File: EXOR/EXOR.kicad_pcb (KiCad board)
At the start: 2 copper layers, 10 parts

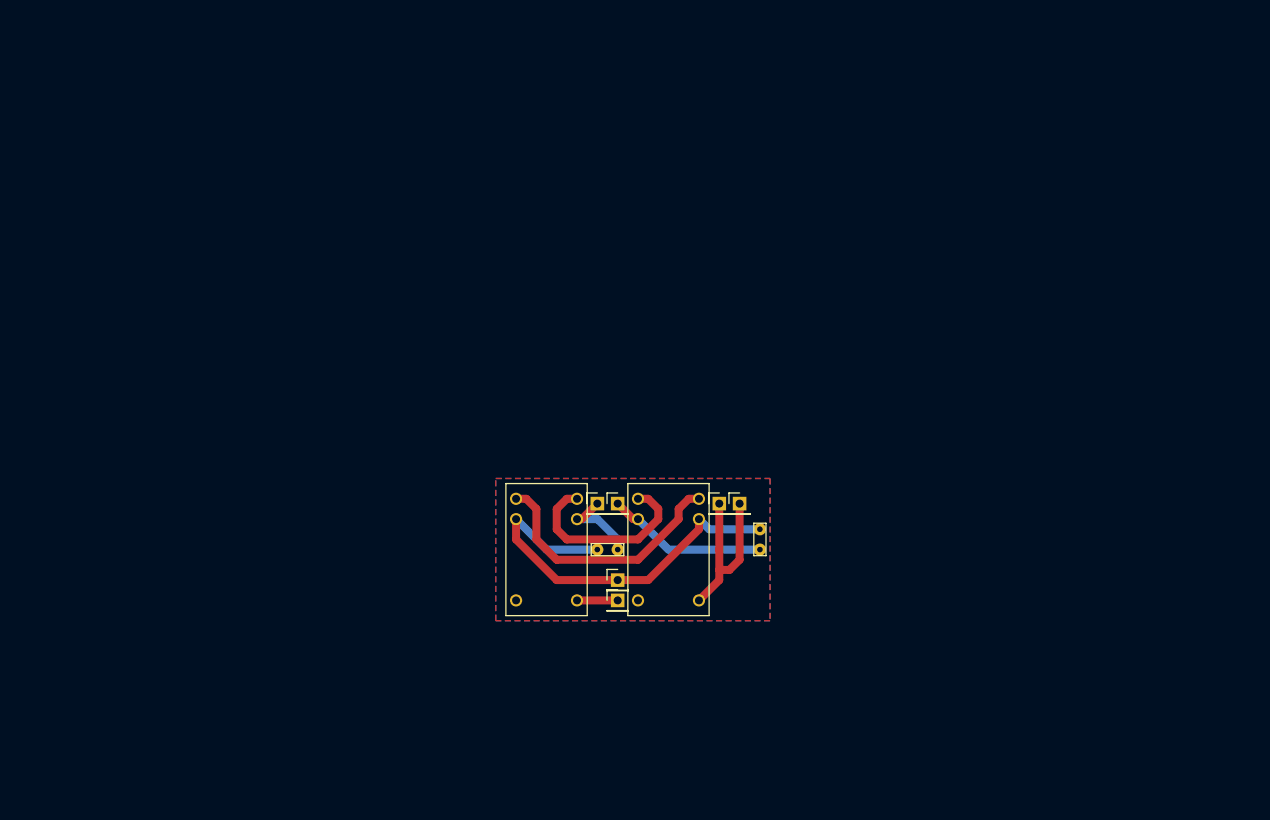
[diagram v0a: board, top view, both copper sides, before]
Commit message: Add files via upload
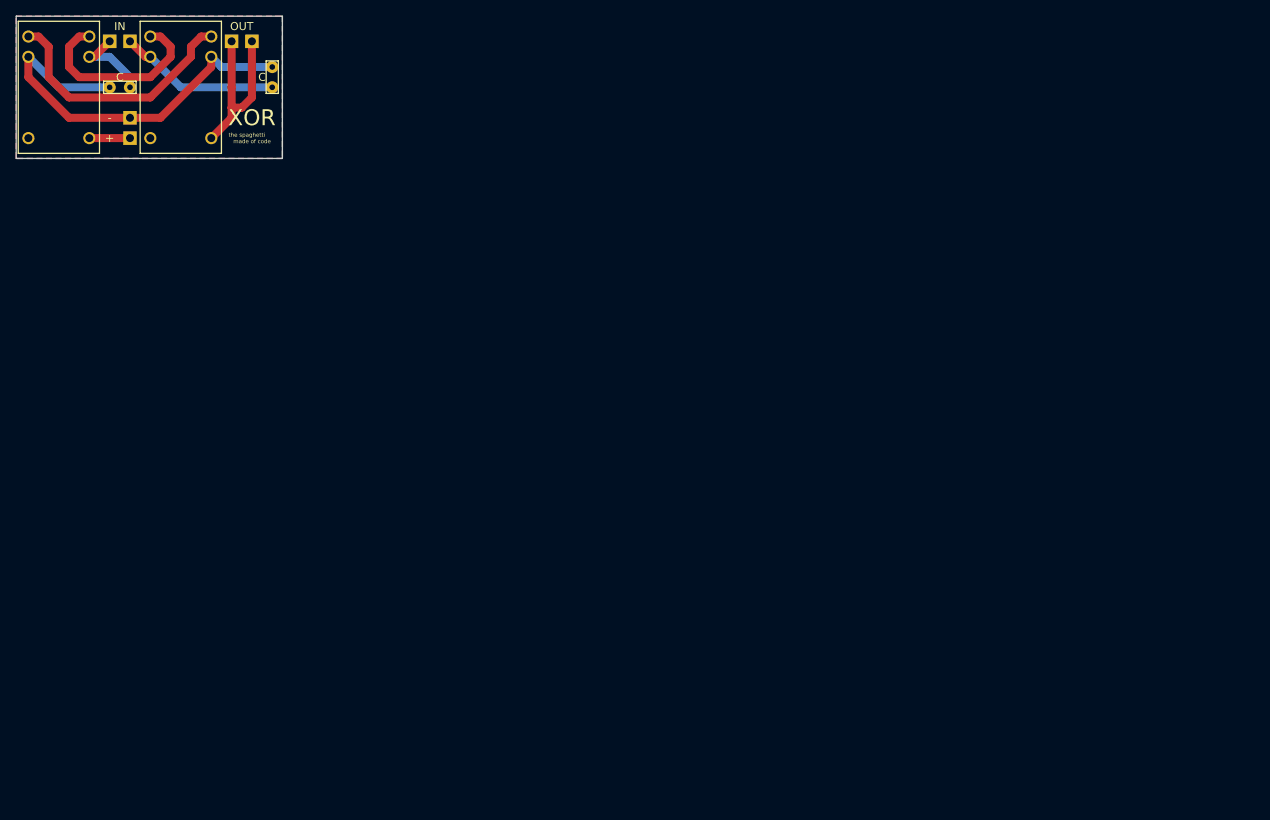
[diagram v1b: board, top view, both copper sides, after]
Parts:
- REF** (x6): moved to B.Cu
- moved REF** 84.0 mm to (45.7, 22.2)
- moved REF** 84.0 mm to (27.9, 26.0)
- moved REF** 84.0 mm to (27.9, 28.6)
- moved REF** 84.0 mm to (27.9, 16.5)
- moved REF** 84.0 mm to (20.3, 21.0)
- moved REF** 84.0 mm to (25.4, 22.2)
- moved REF** 84.0 mm to (43.2, 16.5)
- moved REF** 84.0 mm to (25.4, 16.5)
- moved REF** 84.0 mm to (40.6, 16.5)
- moved REF** 84.0 mm to (35.6, 21.0)
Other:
- board outline added: 33.3 x 17.8 mm
- rule pad_to_mask_clearance: 0.05 -> 0.1
- board text added: "the spaghetti made of code"
- board text removed: "the code made of spaghetti"

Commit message: Add files via upload
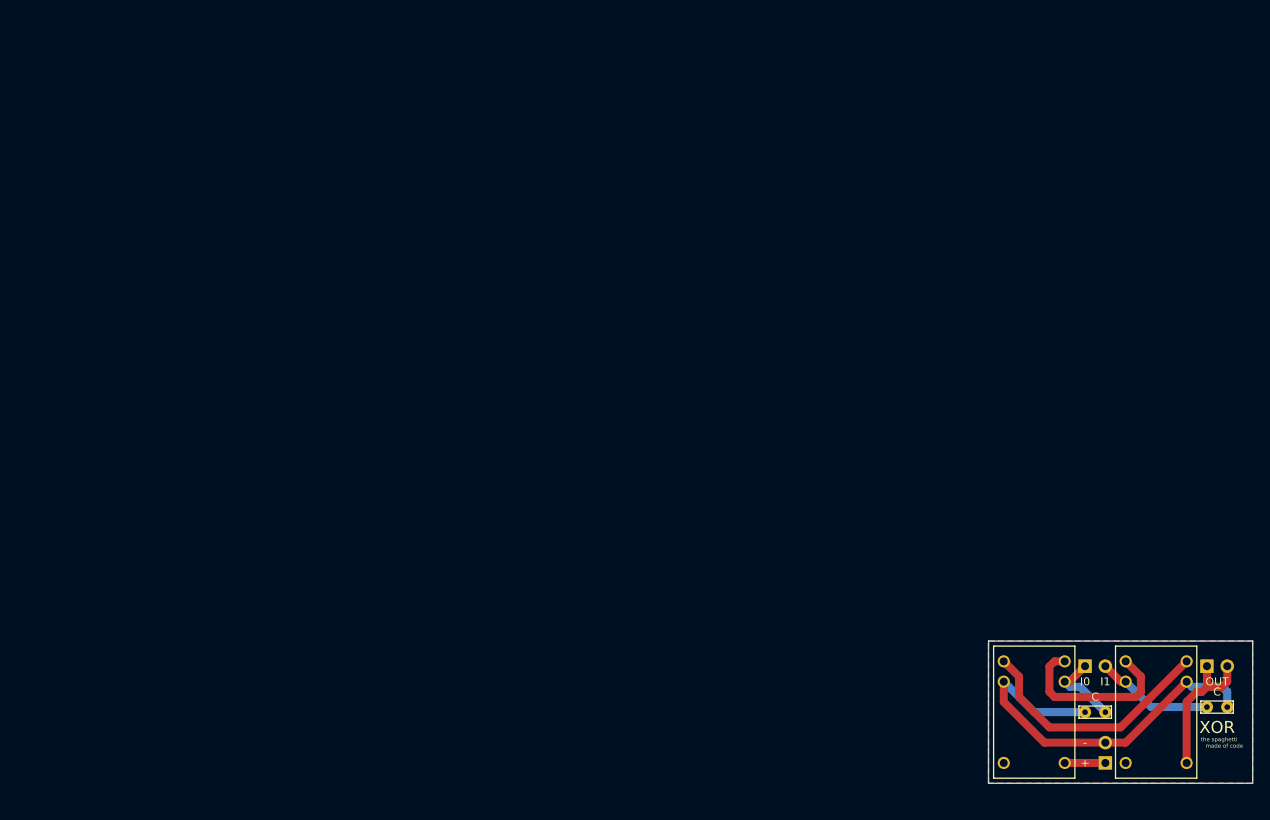
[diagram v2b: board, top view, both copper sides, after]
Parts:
- removed REF** (x2): Condensor, MiyakeFootprintLib:Condensor
- removed REF** (x2): 946H-1C-24D, MiyakeFootprintLib:946H-1C-24D
- removed REF** (x6): PinHeader_1x01_P2.54mm_Vertical, Connector_PinHeader_2.54mm:PinHeader_1x01_P2.54mm_Vertical
- added C1: C, MiyakeFootprintLib:Condensor, F.Cu at (147.3, 100.3)
- added C2: C, MiyakeFootprintLib:Condensor, F.Cu at (162.6, 99.7)
- added J1: Conn_01x02, Connector_PinHeader_2.54mm:PinHeader_1x02_P2.54mm_Vertical, B.Cu at (147.3, 94.6)
- added J2: Conn_01x02, Connector_PinHeader_2.54mm:PinHeader_1x02_P2.54mm_Vertical, B.Cu at (149.9, 106.7)
- added J3: Conn_01x02, Connector_PinHeader_2.54mm:PinHeader_1x02_P2.54mm_Vertical, B.Cu at (162.6, 94.6)
- added SPDT1: 946H-1C-24D, MiyakeFootprintLib:946H-1C-24D, F.Cu at (142.2, 99.1)
- added SPDT2: 946H-1C-24D, MiyakeFootprintLib:946H-1C-24D, F.Cu at (157.5, 99.1)
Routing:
- net (no net): track 166.9 -> 0.00 mm
- net GND: track 0.00 -> 49.9 mm
- net Net-(SPDT1-Pad1): track 0.00 -> 31.2 mm
- net Net-(SPDT1-Pad2): track 0.00 -> 21.9 mm
- net Net-(J3-Pad1): track 0.00 -> 18.3 mm
- net Net-(C2-Pad1): track 0.00 -> 14.8 mm
- net Net-(C1-Pad2): track 0.00 -> 10.0 mm
- net +24V: track 0.00 -> 5.08 mm
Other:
- board size 33.3 x 17.8 mm -> 33 x 17.8 mm
- board text added: "I0"
- board text added: "I1"
- board text removed: "IN"

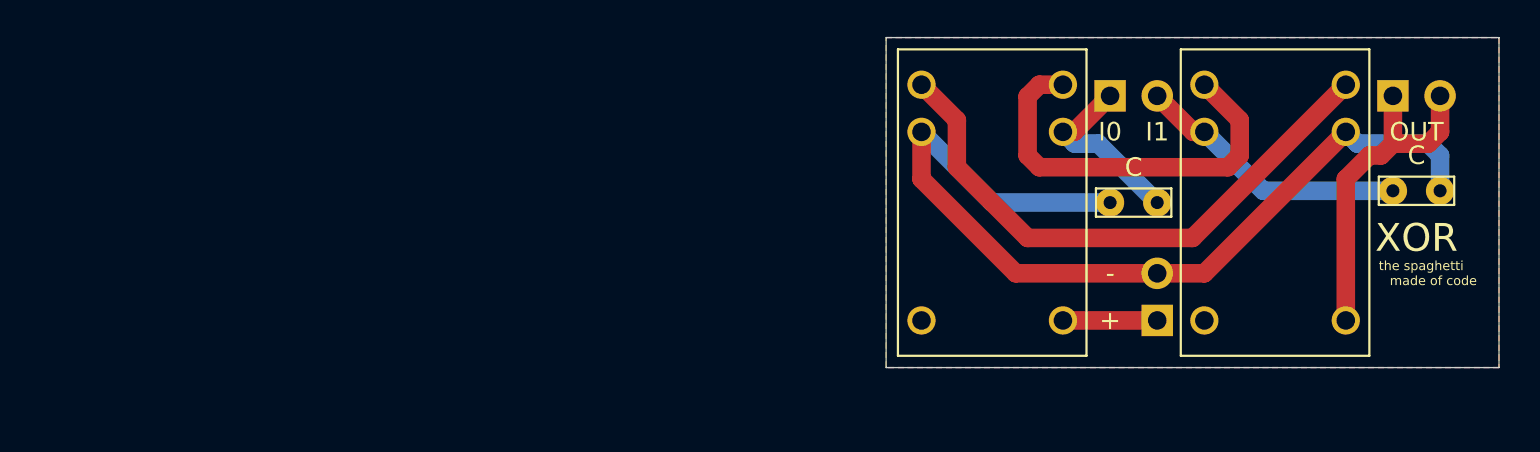
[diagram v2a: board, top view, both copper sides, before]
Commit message: Add files via upload
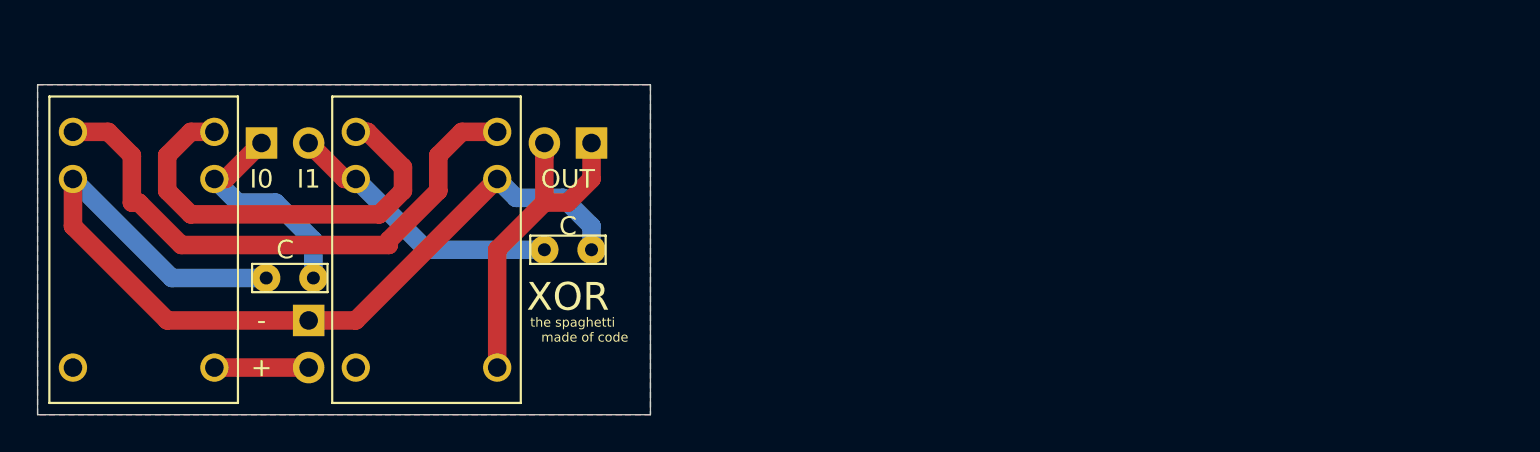
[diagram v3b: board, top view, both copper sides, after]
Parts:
- moved SPDT1 45.8 mm to (96.5, 101.6)
- moved J1 45.8 mm to (101.6, 97.1)
- moved SPDT2 45.8 mm to (111.8, 101.6)
- moved J2 45.7 mm to (104.1, 106.7), turned to 180 degrees
- moved C2 43.3 mm to (119.4, 102.9), turned to 180 degrees
- moved J3 43.3 mm to (119.4, 97.1), turned to 90 degrees
- moved C1 43.1 mm to (104.4, 104.4), turned to 180 degrees
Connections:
- C1 pad 1: GND -> Net-(C1-Pad1)
- C1 pad 2: Net-(C1-Pad2) -> GND
- C2 pad 1: Net-(C2-Pad1) -> GND
- C2 pad 2: GND -> Net-(C2-Pad2)
- J1 pad 1: Net-(C1-Pad2) -> Net-(C1-Pad1)
- J1 pad 2: Net-(C2-Pad1) -> Net-(C2-Pad2)
- J2 pad 1: +24V -> GND
- J2 pad 2: GND -> +24V
- SPDT1 pad 3: Net-(C1-Pad2) -> Net-(C1-Pad1)
- SPDT2 pad 4: Net-(C2-Pad1) -> Net-(C2-Pad2)
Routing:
- net Net-(C2-Pad2): track 0.00 -> 15.1 mm
- net Net-(C2-Pad1): track 14.8 -> 0.00 mm
- net Net-(C1-Pad1): track 0.00 -> 12.1 mm
- net Net-(C1-Pad2): track 10.0 -> 0.00 mm
- net Net-(SPDT1-Pad2): track 21.9 -> 23.3 mm
- net GND: track 49.9 -> 50.7 mm
- net Net-(SPDT1-Pad1): track 31.2 -> 30.7 mm
